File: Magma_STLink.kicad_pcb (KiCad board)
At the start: 2 copper layers, 51.3 x 20.8 mm, 46 parts, among them J1 Conn_01x03, J2 Conn_01x03, J3 Conn_01x02, J4 Conn_01x02, J5 USB_A, U1 LM1117-3.3, U2 STM32F103C8Tx, Y1 Crystal

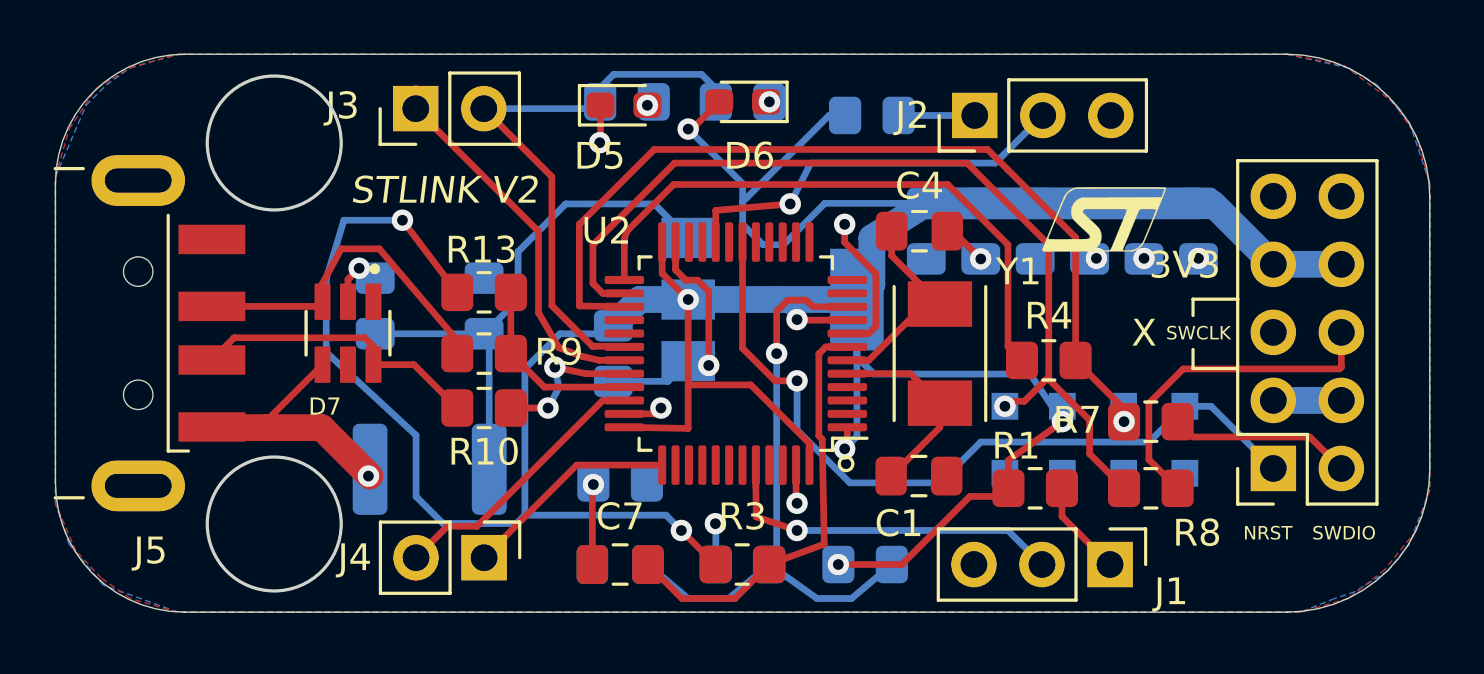
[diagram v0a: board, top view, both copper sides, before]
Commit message: Update project to latest KiCAD version
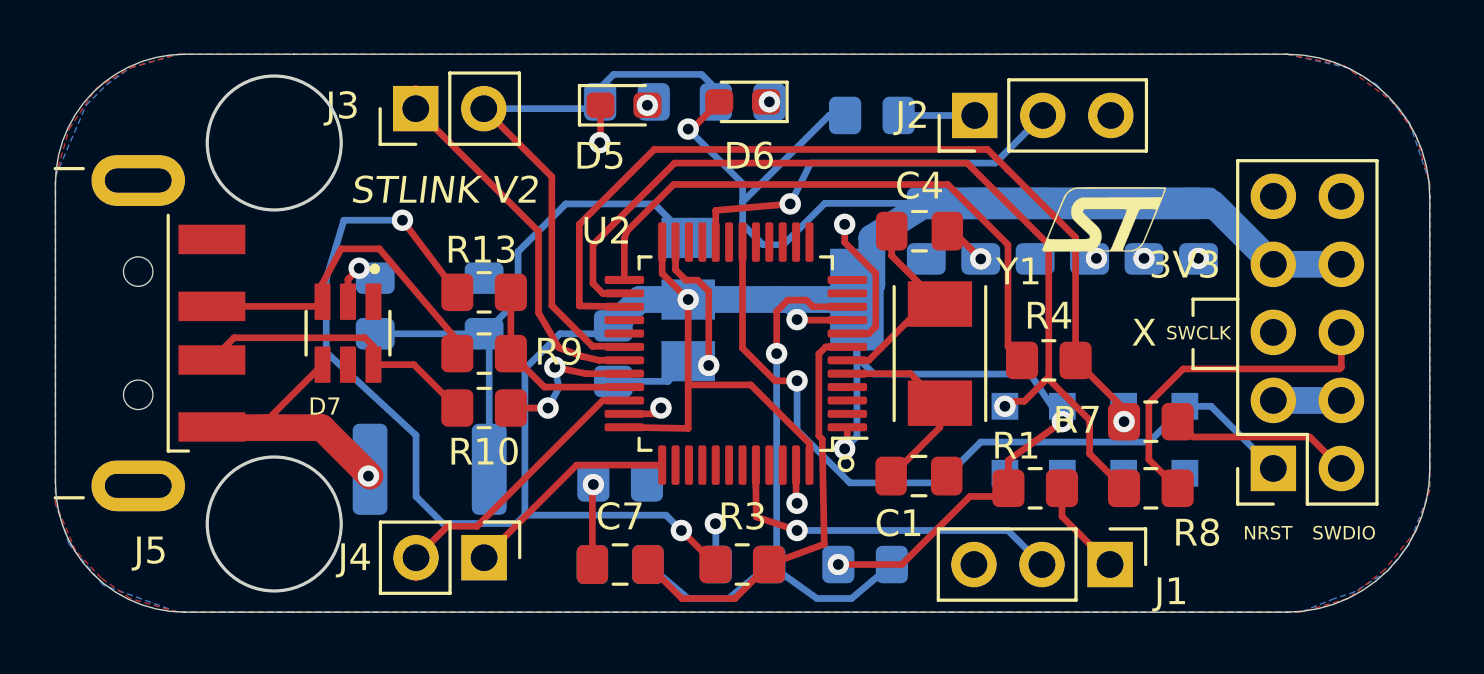
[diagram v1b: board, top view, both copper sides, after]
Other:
- net class Default removed
- net class USB removed
